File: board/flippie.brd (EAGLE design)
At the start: 98.3 x 55.7 mm, 28 parts, among them J1 INT_3V3, U1 FPF2702MX, U10 ULN2803ADW, U11 TD62783AP, U12 TD62783AP, U13 TD62783AP, U14 ULN2803ADW, U2 SN74AHC595D, U3 SN74AHC595D, U4 SN74AHC595D, U5 SN74AHC595D, U6 SN74AHC595D, U7 SN74AHC595D, U8 SN74AHC595D, U9 ULN2803ADW, X1 PWR, X2 BROSE-60-POL

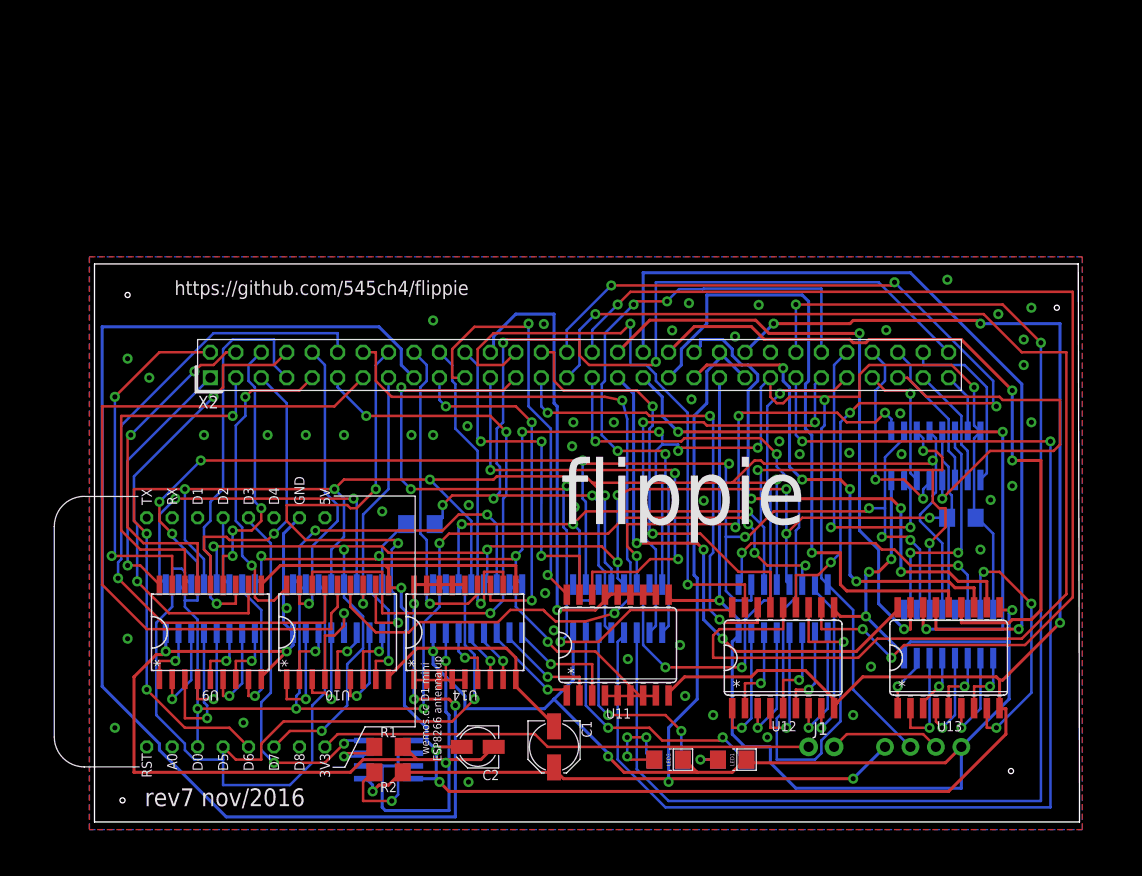
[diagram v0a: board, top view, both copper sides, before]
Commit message: Some clean-ups
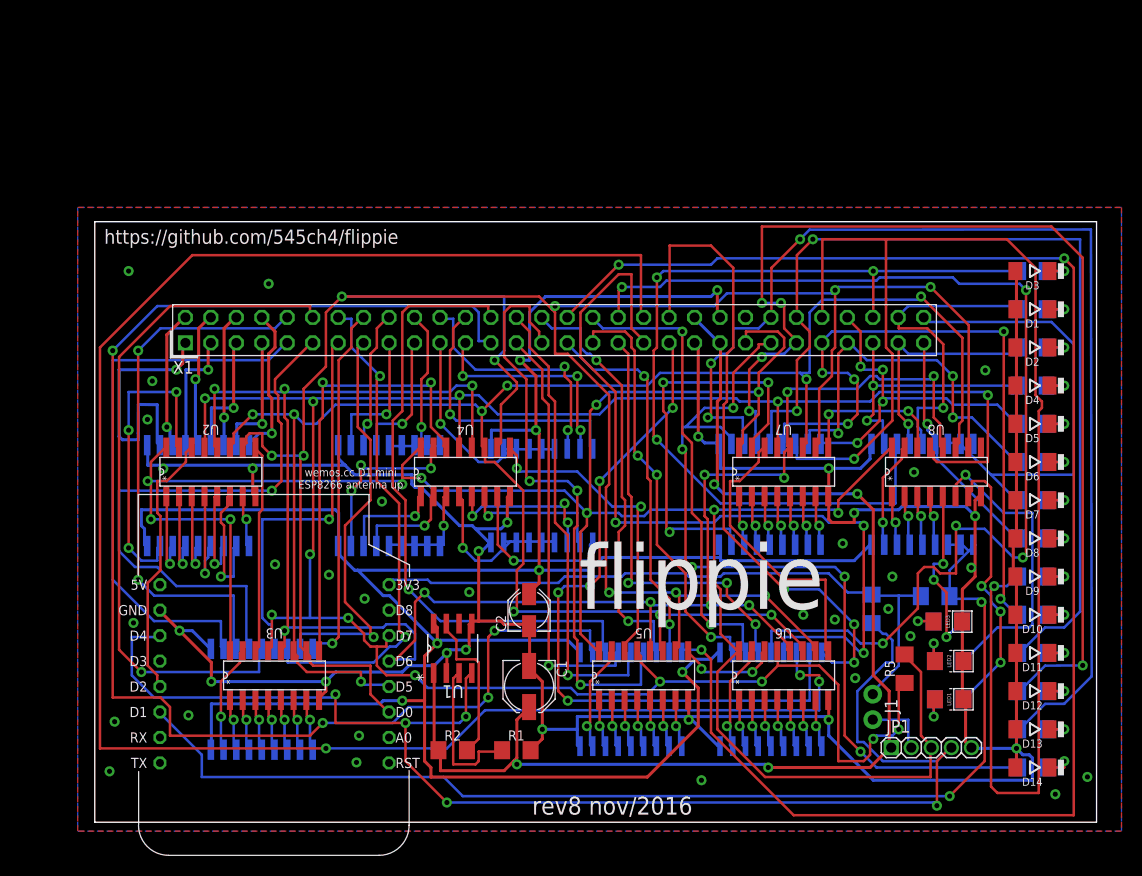
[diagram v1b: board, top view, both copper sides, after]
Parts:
- removed X2: BROSE-60-POL, con-panduit:057-060-1
- added D1, D10, D11, D12, D13, D14, D2, D3, D4, D5, D6, D7, D8, D9: BZV55, diode:SOD80C
- added JP1: (no value), pinhead:1_05X2MM
- added LED3: A, adafruit:1206
- added R10, R11, R12, R13, R14, R15, R16, R17, R18, R19, R20, R21, R22, R9: 100K, rcl:R1206
- added R7, R8: 150, rcl:R1206
- added U15, U16: TD62783AP, uln-udn:SO18W
- LED1: value A -> C
- R4: value 150 -> 10K
- X1: value PWR -> BROSE-60-POL; device adafruit:1X04-CLEANBIG -> con-panduit:057-060-1
- moved U13 76.6 mm to (10.3, 32.6), flipped to the bottom
- moved U9 56.3 mm to (67.5, 12.2), flipped to the bottom
- moved X1 55.5 mm to (45.9, 49.1)
- moved U12 52.2 mm to (16.7, 12.2), flipped to the bottom
- moved R5 50.4 mm to (80.8, 15.3), flipped to the top, turned to 270 degrees
- moved U8 34.6 mm to (84.0, 35.1), flipped to the top
- moved U10 30.0 mm to (53.5, 12.2), flipped to the bottom
- moved LED2 29.7 mm to (85.3, 16.1)
- moved R6 28.6 mm to (85.3, 12.2)
- moved U11 27.2 mm to (29.4, 32.6), flipped to the bottom
- moved LED1 22.5 mm to (85.3, 12.2)
- moved R4 20.5 mm to (77.5, 21.3), turned to 270 degrees
- moved MCU1 17.4 mm to (29.4, 23.7), turned to 180 degrees
- moved U6 17.0 mm to (68.8, 14.8), flipped to the top
- moved U14 15.6 mm to (44.6, 32.6), flipped to the bottom
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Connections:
- removed net SR10_ROW15_24V: U10.12, X2.15
- removed net SR11_ROW14_24V: U10.13, X2.14
- removed net SR12_ROW13_24V: U10.14, X2.13
- removed net SR13_ROW12_24V: U10.15, X2.12
- removed net SR14_ROW11_24V: U10.16, X2.11
- removed net SR15_ROW10_24V: U10.17, X2.10
- removed net SR16_ROW9_24V: U10.18, X2.9
- removed net SR17_ROW4_GND: U11.11, U11.12, U11.13, U11.14, U11.15, X2.24
- removed net SR18_ROW3_GND: U11.16, X2.23
- removed net SR19_ROW2_GND: U11.17, X2.22
- removed net SR1_ROW8_24V: U9.11, X2.8
- removed net SR20_ROW1_GND: U11.18, X2.21
- removed net SR21_ROW20_24V: U14.11, X2.20
- removed net SR22_ROW19_24V: U14.12, X2.19
- removed net SR23_ROW18_24V: U14.13, X2.18
- removed net SR24_ROW17_24V: U14.14, U14.15, U14.16, U14.17, U14.18, X2.17
- removed net SR25_ROW12_GND: U12.11, X2.32
- removed net SR26_ROW11_GND: U12.12, X2.31
- removed net SR27_ROW10_GND: U12.13, X2.30
- removed net SR28_ROW9_GND: U12.14, X2.29
- removed net SR29_ROW8_GND: U12.15, X2.28
- removed net SR2_ROW7_24V: U9.12, X2.7
- removed net SR30_ROW7_GND: U12.16, X2.27
- removed net SR31_ROW6_GND: U12.17, X2.26
- removed net SR32_ROW5_GND: U12.18, X2.25
- removed net SR33_ROW20_GND: U13.11, X2.40
- removed net SR34_ROW19_GND: U13.12, X2.39
- removed net SR35_ROW18_GND: U13.13, X2.38
- removed net SR36_ROW17_GND: U13.14, X2.37
- removed net SR37_ROW16_GND: U13.15, X2.36
- removed net SR38_ROW15_GND: U13.16, X2.35
- removed net SR39_ROW14_GND: U13.17, X2.34
- removed net SR3_ROW6_24V: U9.13, X2.6
- removed net SR40_ROW13_GND: U13.18, X2.33
- removed net SR41_ADDR7: U7.15, X2.59
- removed net SR42_ADDR6: U7.1, X2.58
- removed net SR43_ADDR5: U7.2, X2.57
- removed net SR44_ADDR4: U7.3, X2.56
- removed net SR45_ADDR3: U7.4, X2.55
- removed net SR46_ADDR2: U7.5, X2.54
- removed net SR47_ADDR1: U7.6, X2.53
- removed net SR48_B1@FP2800A: U7.7, X2.52
- removed net SR49_B0@FP2800A: U8.15, X2.51
- removed net SR4_ROW5_24V: U9.14, X2.5
- removed net SR50_A2@FP2800A: U8.1, X2.50
- removed net SR51_A1@FP2800A: U8.2, X2.49
- removed net SR52_A0@FP2800A: U8.3, X2.48
- removed net SR53_D@FP2800A: U8.4, X2.47
- removed net SR54_ADDR8_NOT_EN: R5.1, U8.5, X2.60
- removed net SR56_LED_A: R4.1, U8.7
- removed net SR5_ROW4_24V: U9.15, X2.4
- removed net SR6_ROW3_24V: U9.16, X2.3
- removed net SR7_ROW2_24V: U9.17, X2.2
- removed net SR8_ROW1_24V: U9.18, X2.1
- removed net SR9_ROW16_24V: U10.11, X2.16
- new net N$10: D6.C, R14.2
- new net N$12: D7.C, R15.2
- new net N$13: D8.C, R16.2
- new net N$14: D9.C, R17.2
- new net N$15: D10.C, R18.2
- new net N$16: D11.C, R19.2
- new net N$17: D12.C, R20.2
- new net N$18: D13.C, R21.2
- new net N$19: D14.C, R22.2
- new net N$2: D1.C, R9.2
- new net N$5: LED3.A, R8.2
- new net N$6: D2.C, R10.2
- new net N$7: D3.C, R11.2
- new net N$8: D4.C, R12.2
- new net N$9: D5.C, R13.2
- new net NOT_EN_ADDR8@FP2800A: MCU1.D1, R3.2, U15.1, U15.2, U15.3
- new net NOT_EN_ADDR8@FP2800A_VS: R15.1, U15.16, U15.17, U15.18, X1.60
- new net SR10_ROW10_SET: U12.12, X1.10
- new net SR11_ROW11_SET: U12.13, X1.11
- new net SR12_ROW12_SET: U12.14, X1.12
- new net SR13_ROW13_SET: U12.15, X1.13
- new net SR14_ROW14_SET: U12.16, X1.14
- new net SR15_ROW15_SET: U12.17, X1.15
- new net SR16_ROW16_SET: U12.18, X1.16
- new net SR17_ROW17_SET: U11.11, X1.17
- new net SR18_ROW18_SET: U11.12, X1.18
- new net SR19_ROW19_SET: U11.13, X1.19
- new net SR1_ROW1_SET: U13.11, X1.1
- new net SR20_ROW20_SET: U11.14, U11.15, U11.16, U11.17, U11.18, X1.20
- new net SR21_ROW1_RST: U14.11, U14.12, U14.13, U14.14, U14.15, X1.21
- new net SR22_ROW2_RST: U14.16, X1.22
- new net SR23_ROW3_RST: U14.17, X1.23
- new net SR24_ROW4_RST: U14.18, X1.24
- new net SR25_ROW5_RST: U10.11, X1.25
- new net SR26_ROW6_RST: U10.12, X1.26
- new net SR27_ROW7_RST: U10.13, X1.27
- new net SR28_ROW8_RST: U10.14, X1.28
- new net SR29_ROW9_RST: U10.15, X1.29
- new net SR2_ROW2_SET: U13.12, X1.2
- new net SR30_ROW10_RST: U10.16, X1.30
- new net SR31_ROW11_RST: U10.17, X1.31
- new net SR32_ROW12_RST: U10.18, X1.32
- new net SR33_ROW13_RST: U9.11, X1.33
- new net SR34_ROW14_RST: U9.12, X1.34
- new net SR35_ROW15_RST: U9.13, X1.35
- new net SR36_ROW16_RST: U9.14, X1.36
- new net SR37_ROW17_RST: U9.15, X1.37
- new net SR38_ROW18_RST: U9.16, X1.38
- new net SR39_ROW19_RST: U9.17, X1.39
- new net SR3_ROW3_SET: U13.13, X1.3
- new net SR40_ROW20_RST: U9.18, X1.40
- new net SR41_D@FP2800A: U16.8, U7.15
- new net SR41_D@FP2800A_VS: R22.1, U16.11, X1.47
- new net SR42_A0@FP2800A: U16.7, U7.1
- new net SR42_A0@FP2800A_VS: R21.1, U16.12, X1.48
- new net SR43_A1@FP2800A: U16.6, U7.2
- new net SR43_A1@FP2800A_VS: R20.1, U16.13, X1.49
- new net SR44_A2@FP2800A: U16.5, U7.3
- new net SR44_A2@FP2800A_VS: R19.1, U16.14, X1.50
- new net SR45_B0@FP2800A: U16.4, U7.4
- new net SR45_B0@FP2800A_VS: R18.1, U16.15, X1.51
- new net SR46_B1@FP2800A: U16.3, U7.5
- new net SR46_B1@FP2800A_VS: R17.1, U16.16, X1.52
- new net SR47_ADDR1@FP2800A: U16.2, U7.6
- new net SR47_ADDR1@FP2800A_VS: R14.1, U16.17, X1.53
- new net SR48_ADDR2@FP2800A: U16.1, U7.7
- new net SR48_ADDR2@FP2800A_VS: R13.1, U16.18, X1.54
- new net SR49_ADDR3@FP2800A: U15.8, U8.15
- new net SR49_ADDR3@FP2800A_VS: R12.1, U15.11, X1.55
- new net SR4_ROW4_SET: U13.14, X1.4
- new net SR50_ADDR4@FP2800A: U15.7, U8.1
- new net SR50_ADDR4@FP2800A_VS: R11.1, U15.12, X1.56
- new net SR51_ADDR5@FP2800A: U15.6, U8.2
- new net SR51_ADDR5@FP2800A_VS: R10.1, U15.13, X1.57
- new net SR52_ADDR6@FP2800A: U15.5, U8.3
- new net SR52_ADDR6@FP2800A_VS: R9.1, U15.14, X1.58
- new net SR53_ADDR7@FP2800A: U15.4, U8.4
- new net SR53_ADDR7@FP2800A_VS: R16.1, U15.15, X1.59
- new net SR54_LED_A: R8.1, U8.5
- new net SR56_LED_C: R6.1, U8.7
- new net SR5_ROW5_SET: U13.15, X1.5
- new net SR6_ROW6_SET: U13.16, X1.6
- new net SR7_ROW7_SET: U13.17, X1.7
- new net SR8_ROW8_SET: U13.18, X1.8
- new net SR9_ROW9_SET: U12.11, X1.9
- net +24V: now also JP1.1, X1.42, X1.43; no longer X1.1, X2.42, X2.43
- net +3V3: now also JP1.3; no longer X1.3
- net +3V3_SW: now also R3.1, R4.1
- net +5V: now also JP1.2, R5.1, X1.45; no longer R3.1, R5.2, X1.2, X2.45
- net +VS: now also U15.9, U16.9, X1.44; no longer X2.44
- net EN_VS: now also JP1.4, MCU1.D4, R4.2; no longer MCU1.D3
- net GND: now also D1.A, D10.A, D11.A, D12.A, D13.A, D14.A, D2.A, D3.A, D4.A, D5.A, D6.A, D7.A, D8.A, D9.A, JP1.5, LED3.C, U15.10, U16.10, X1.41; no longer X1.4, X2.41
- net N$142: now also R7.2; no longer R6.2
- net N$148: now also R6.2; no longer R4.2
- net SR1: now also U13.8; no longer U9.8
- net SR10: now also U12.7; no longer U10.7
- net SR11: now also U12.6; no longer U10.6
- net SR12: now also U12.5; no longer U10.5
- net SR13: now also U12.4; no longer U10.4
- net SR14: now also U12.3; no longer U10.3
- net SR15: now also U12.2; no longer U10.2
- net SR16: now also U12.1; no longer U10.1
- net SR17: no longer U11.4, U11.5, U11.6, U11.7
- net SR18: now also U11.7; no longer U11.3
- net SR19: now also U11.6; no longer U11.2
- net SR2: now also U13.7; no longer U9.7
- net SR20: now also U11.2, U11.3, U11.4, U11.5
- net SR21: now also U14.4, U14.5, U14.6, U14.7
- net SR22: now also U14.3; no longer U14.7
- net SR23: now also U14.2; no longer U14.6
- net SR24: no longer U14.2, U14.3, U14.4, U14.5
- net SR25: now also U10.8; no longer U12.8
- net SR26: now also U10.7; no longer U12.7
- net SR27: now also U10.6; no longer U12.6
- net SR28: now also U10.5; no longer U12.5
- net SR29: now also U10.4; no longer U12.4
- net SR3: now also U13.6; no longer U9.6
- net SR30: now also U10.3; no longer U12.3
- net SR31: now also U10.2; no longer U12.2
- net SR32: now also U10.1; no longer U12.1
- net SR33: now also U9.8; no longer U13.8
- net SR34: now also U9.7; no longer U13.7
- net SR35: now also U9.6; no longer U13.6
- net SR36: now also U9.5; no longer U13.5
- net SR37: now also U9.4; no longer U13.4
- net SR38: now also U9.3; no longer U13.3
- net SR39: now also U9.2; no longer U13.2
- net SR4: now also U13.5; no longer U9.5
- net SR40: now also U9.1; no longer U13.1
- net SR5: now also U13.4; no longer U9.4
- net SR55_LED_B: now also R7.1; no longer R6.1
- net SR6: now also U13.3; no longer U9.3
- net SR7: now also U13.2; no longer U9.2
- net SR8: now also U13.1; no longer U9.1
- net SR9: now also U12.8; no longer U10.8
- net ~OE: now also R5.2; no longer R3.2
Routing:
- net SR38_ROW18_RST: track 0.00 -> 185.5 mm, vias 0 -> 3
- net SR32_ROW12_RST: track 0.00 -> 158.5 mm, vias 0 -> 3
- net SR24_ROW17_24V: track 143.4 -> 0.00 mm, vias 3 -> 0
- net SR46_B1@FP2800A_VS: track 0.00 -> 142.0 mm, vias 0 -> 2
- net SR25_ROW5_RST: track 0.00 -> 138.4 mm, vias 0 -> 4
- net SR52_A0@FP2800A: track 131.8 -> 0.00 mm, vias 2 -> 0
- net SR28_ROW9_GND: track 129.7 -> 0.00 mm, vias 1 -> 0
- net SR53_D@FP2800A: track 126.0 -> 0.00 mm, vias 2 -> 0
- net NOT_EN_ADDR8@FP2800A: track 0.00 -> 116.8 mm, vias 0 -> 2
- net SR42_A0@FP2800A_VS: track 0.00 -> 113.2 mm, vias 0 -> 3
- net SR25_ROW12_GND: track 113.2 -> 0.00 mm, vias 3 -> 0
- net SR36_ROW16_RST: track 0.00 -> 110.5 mm, vias 0 -> 5
- net SR43_A1@FP2800A_VS: track 0.00 -> 109.6 mm, vias 0 -> 5
- net SR54_ADDR8_NOT_EN: track 106.2 -> 0.00 mm, vias 5 -> 0
- net EN_VS: track 36.4 -> 139.3 mm, vias 2 -> 5
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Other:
- board size 98.3 x 55.7 mm -> 99.9 x 59.9 mm
- board text added: "EN+"
- board text added: "rev8 nov/2016"
- board text removed: "rev7 nov/2016"

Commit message: Update board to rev10
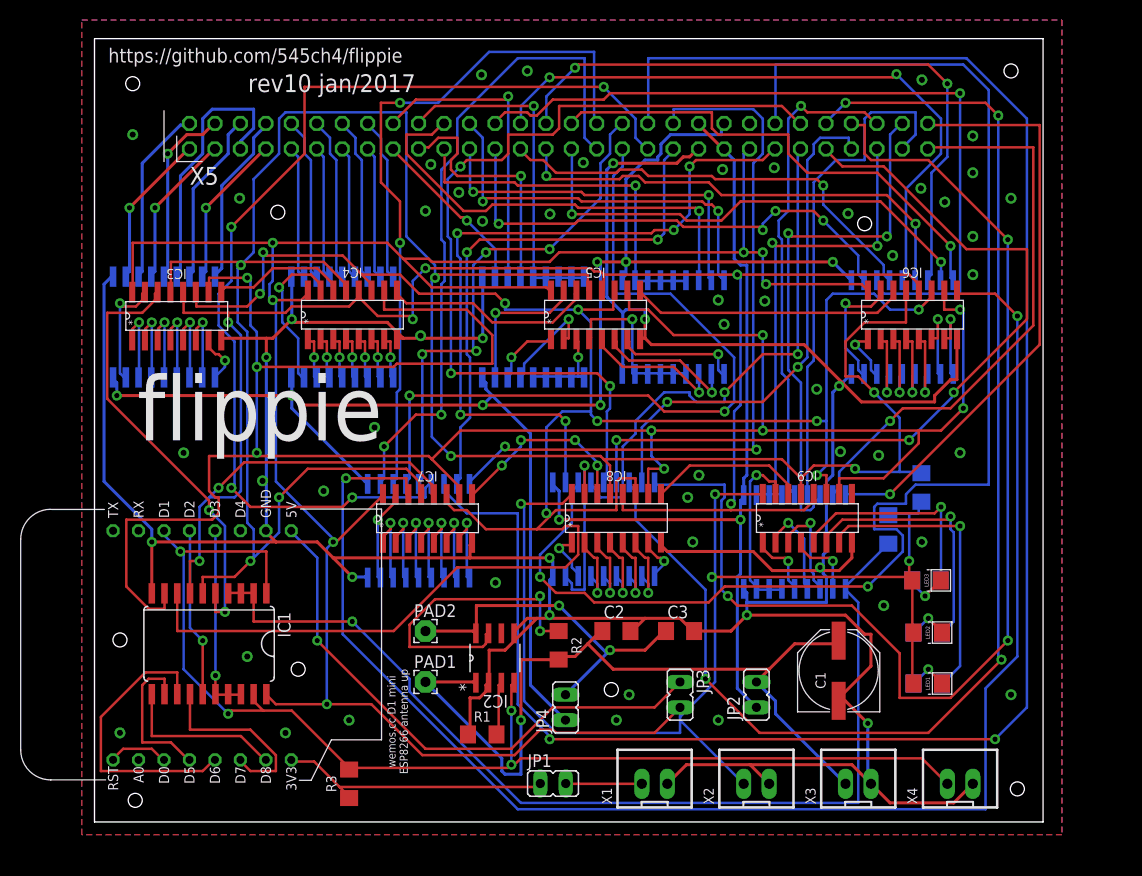
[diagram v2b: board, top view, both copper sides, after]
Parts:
- removed D1, D10, D11, D12, D13, D14, D2, D3, D4, D5, D6, D7, D8, D9: BZV55, diode:SOD80C
- removed J1: INT_3V3, SparkFun-Connectors:1X02_NO_SILK
- removed R10, R11, R12, R13, R14, R15, R16, R17, R18, R19, R20, R21, R22, R9: 100K, rcl:R1206
- removed U1: FPF2702MX, ON Semiconductor_By_element14_Batch_1:SOIC127P600X175-8N
- removed U10, U14, U9: ULN2803ADW, Texas Instruments_By_element14_Batch_1:SOIC127P1030X265-18N
- removed U11, U12, U13, U15, U16: TD62783AP, uln-udn:SO18W
- removed U2, U3, U4, U5, U6, U7, U8: SN74AHC595D, Texas Instruments_By_element14_Batch_1:SOIC127P600X175-16N
- added C3: 22u, rcl:C1206
- added IC1: 74HCT245DW, 74xx-eu:SO20W
- added IC10, IC11, IC12: TD62783AFG, uln-udn:SO18W
- added IC13, IC14, IC15, IC16, IC17: ULN2803A, Texas Instruments_By_element14_Batch_1:SOIC127P1030X265-18N
- added IC2: FPF2702MX, ON Semiconductor_By_element14_Batch_1:SOIC127P600X175-8N
- added IC3, IC4, IC5, IC6, IC7, IC8, IC9: SN74AHC595D, Texas Instruments_By_element14_Batch_1:SOIC127P600X175-16N
- added JP2: 24V, jumper:JP1
- added JP3: 5V, jumper:JP1
- added JP4: VS, jumper:JP1
- added PAD1: 24V, wirepad:2,15/1,0
- added PAD2: VS, wirepad:2,15/1,0
- added X2: 5V, Rembrandt Electronics - JST XH Connectors v1-0:JST-XH-02-PACKAGE-LONG-PAD
- added X3: 24V, Rembrandt Electronics - JST XH Connectors v1-0:JST-XH-02-PACKAGE-LONG-PAD
- added X4: ~EN_PWR, Rembrandt Electronics - JST XH Connectors v1-0:JST-XH-02-PACKAGE-LONG-PAD
- added X5: BROSE-60-POL, con-panduit:057-060-1
- C1: value 100u -> 100u/35V; device rcl:PANASONIC_C -> rcl:PANASONIC_E
- C2: value 22u -> 100u; device rcl:PANASONIC_B -> rcl:C1206
- JP1: value (none) -> 3V3; device pinhead:1_05X2MM -> jumper:JP1
- LED1: value C -> C (red)
- LED2: value B -> B (yellow)
- LED3: value A -> A (green)
- R1: value 680K -> 470K
- R6: value 150 -> 180
- R8: value 150 -> 120
- X1: value BROSE-60-POL -> 3V3; device con-panduit:057-060-1 -> Rembrandt Electronics - JST XH Connectors v1-0:JST-XH-02-PACKAGE-LONG-PAD
- moved R3 61.4 mm to (25.4, 3.81), flipped to the top, turned to 90 degrees
- moved X1 46.4 mm to (55.9, 3.81)
- moved JP1 37.9 mm to (45.7, 3.84), turned to 270 degrees
- moved C1 30.9 mm to (74.2, 15.1), turned to 90 degrees
- moved MCU1 20.0 mm to (19.6, 6.20), turned to 90 degrees
- moved R5 18.2 mm to (82.5, 33.4), flipped to the bottom, turned to 90 degrees
- moved R2 14.9 mm to (46.3, 17.6), turned to 270 degrees
- moved C2 8.96 mm to (52.1, 19.1), turned to 0 degrees
- moved R4 8.10 mm to (79.2, 29.2)
- moved LED3 4.64 mm to (83.0, 24.1)
- moved R8 4.64 mm to (83.0, 24.1)
- moved R1 3.75 mm to (38.7, 8.74), turned to 0 degrees
- moved LED2 3.56 mm to (83.1, 18.9)
- moved R7 3.56 mm to (83.1, 18.9)
- moved LED1 2.65 mm to (83.1, 13.8)
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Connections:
- removed net +24V: C1.+, JP1.1, R2.2, U1.1, X1.42, X1.43
- removed net +3V3: J1.2, JP1.3
- removed net +3V3_SW: J1.1, MCU1.3V3, R3.1, R4.1
- removed net +5V: JP1.2, R5.1, U2.16, U3.16, U4.16, U5.16, U6.16, U7.16, U8.16, X1.45
- removed net +VS: C2.+, U1.8, U10.10, U11.9, U12.9, U13.9, U14.10, U15.9, U16.9, U9.10, X1.44
- removed net EN_VS: JP1.4, MCU1.D4, R4.2, U1.4
- removed net N$10: D6.C, R14.2
- removed net N$12: D7.C, R15.2
- removed net N$13: D8.C, R16.2
- removed net N$14: D9.C, R17.2
- removed net N$142: LED2.A, R7.2
- removed net N$148: LED1.A, R6.2
- removed net N$15: D10.C, R18.2
- removed net N$16: D11.C, R19.2
- removed net N$17: D12.C, R20.2
- removed net N$18: D13.C, R21.2
- removed net N$19: D14.C, R22.2
- removed net N$2: D1.C, R9.2
- removed net N$41: U7.9, U8.14
- removed net N$6: D2.C, R10.2
- removed net N$9: D5.C, R13.2
- removed net NOT_EN_ADDR8@FP2800A: MCU1.D1, R3.2, U15.1, U15.2, U15.3
- removed net NOT_EN_ADDR8@FP2800A_VS: R15.1, U15.16, U15.17, U15.18, X1.60
- removed net SR41_D@FP2800A_VS: R22.1, U16.11, X1.47
- removed net SR42_A0@FP2800A_VS: R21.1, U16.12, X1.48
- removed net SR43_A1@FP2800A_VS: R20.1, U16.13, X1.49
- removed net SR44_A2@FP2800A_VS: R19.1, U16.14, X1.50
- removed net SR45_B0@FP2800A_VS: R18.1, U16.15, X1.51
- removed net SR46_B1@FP2800A_VS: R17.1, U16.16, X1.52
- removed net SR47_ADDR1@FP2800A_VS: R14.1, U16.17, X1.53
- removed net SR48_ADDR2@FP2800A_VS: R13.1, U16.18, X1.54
- removed net SR49_ADDR3@FP2800A_VS: R12.1, U15.11, X1.55
- removed net SR50_ADDR4@FP2800A_VS: R11.1, U15.12, X1.56
- removed net SR51_ADDR5@FP2800A_VS: R10.1, U15.13, X1.57
- removed net SR52_ADDR6@FP2800A_VS: R9.1, U15.14, X1.58
- removed net SR53_ADDR7@FP2800A_VS: R16.1, U15.15, X1.59
- new net 24V: IC16.10, IC17.10, JP2.1, X5.42, X5.43
- new net 24V_SW: C1.+, C2.1, IC2.1, JP2.2, PAD1.1, R2.2, X3.1
- new net 3V3: JP1.2, X1.1
- new net 3V3_SW: JP1.1, MCU1.3V3, R3.1
- new net N$21: LED2.C, R7.2
- new net N$23: LED3.C, R8.2
- new net RCLK_5V: IC1.7, IC3.12, IC4.12, IC5.12, IC6.12, IC7.12, IC8.12, IC9.12
- new net SER_5V: IC1.5, IC3.14
- new net SR41_D@FP2800A_24V: IC17.11, X5.47
- new net SR42_A0@FP2800A_24V: IC17.12, X5.48
- new net SR43_A1@FP2800A_24V: IC17.13, X5.49
- new net SR44_A2@FP2800A_24V: IC17.14, X5.50
- new net SR45_B0@FP2800A_24V: IC17.15, X5.51
- new net SR46_B1@FP2800A_24V: IC17.16, X5.52
- new net SR47_ADDR1@FP2800A_24V: IC17.17, X5.53
- new net SR48_ADDR2@FP2800A_24V: IC17.18, X5.54
- new net SR49_ADDR3@FP2800A_24V: IC16.11, IC16.12, IC16.13, X5.55
- new net SR50_ADDR4@FP2800A_24V: IC16.14, X5.56
- new net SR51_ADDR5@FP2800A_24V: IC16.15, X5.57
- new net SR52_ADDR6@FP2800A_24V: IC16.16, X5.58
- new net SR53_ADDR7@FP2800A_24V: IC16.17, X5.59
- new net SRCLK_5V: IC1.8, IC3.11, IC4.11, IC5.11, IC6.11, IC7.11, IC8.11, IC9.11
- new net VCC: IC1.20, IC3.16, IC4.16, IC5.16, IC6.16, IC7.16, IC8.16, IC9.16, JP3.2, LED1.A, LED2.A, LED3.A, R4.1, R5.1, X2.1, X5.45
- new net VCC_SW: JP3.1, MCU1.5V
- new net VS: IC10.9, IC11.9, IC12.9, IC13.10, IC14.10, IC15.10, JP4.1, X5.44
- new net VS_SW: C3.1, IC2.8, JP4.2, PAD2.1
- new net ~EN_ADDR8@FP2800A: IC1.16, IC1.17, IC1.18, MCU1.D3
- new net ~EN_ADDR8@FP2800A_24V: IC16.18, X5.60
- new net ~EN_ADDR8@FP2800A_5V: IC1.2, IC1.3, IC1.4, IC16.1, R4.2
- new net ~EN_POWER_RAILS: IC1.1, IC1.19, IC2.4, MCU1.D1, R3.2, X4.1
- new net ~OE_5V: IC1.6, IC3.13, IC4.13, IC5.13, IC6.13, IC7.13, IC8.13, IC9.13, R5.2
- new net ~SRCLR_5V: IC1.9, IC3.10, IC4.10, IC5.10, IC6.10, IC7.10, IC8.10, IC9.10
- net GND: now also C2.2, C3.2, IC1.10, IC10.10, IC11.10, IC12.10, IC13.9, IC14.9, IC15.9, IC16.9, IC17.9, IC2.2, IC2.5, IC3.8, IC4.8, IC5.8, IC6.8, IC7.8, IC8.8, IC9.8, X1.2, X2.2, X3.2, X4.2, X5.41; no longer C2.-, D1.A, D10.A, D11.A, D12.A, D13.A, D14.A, D2.A, D3.A, D4.A, D5.A, D6.A, D7.A, D8.A, D9.A, JP1.5, LED1.C, LED2.C, LED3.C, U1.2, U1.5, U10.9, U11.10, U12.10, U13.10, U14.9, U15.10, U16.10, U2.8, U3.8, U4.8, U5.8, U6.8, U7.8, U8.8, U9.9, X1.41
- net N$1: now also IC6.9, IC7.14; no longer U5.9, U6.14
- net N$11: now also IC4.9, IC5.14; no longer U3.9, U4.14
- net N$22: now also IC5.9, IC6.14; no longer U4.9, U5.14
- net N$3: now also IC2.7; no longer U1.7
- net N$31: now also IC3.9, IC4.14; no longer U2.9, U3.14
- net N$37: now also IC7.9, IC8.14; no longer U6.9, U7.14
- net N$4: now also IC2.3; no longer U1.3
- net N$5: now also LED1.C, R6.2; no longer LED3.A, R8.2
- net N$7: now also IC8.9, IC9.14; no longer D3.C, R11.2
- net N$8: now also MCU1.D0, MCU1.RST; no longer D4.C, R12.2
- net RCLK: now also IC1.13; no longer U2.12, U3.12, U4.12, U5.12, U6.12, U7.12, U8.12
- net SER: now also IC1.15; no longer U2.14
- net SR1: now also IC12.8, IC3.15; no longer U13.8, U2.15
- net SR10: now also IC11.7, IC4.1; no longer U12.7, U3.1
- net SR10_ROW10_SET: now also IC11.12, X5.10; no longer U12.12, X1.10
- net SR11: now also IC11.6, IC4.2; no longer U12.6, U3.2
- net SR11_ROW11_SET: now also IC11.13, X5.11; no longer U12.13, X1.11
- net SR12: now also IC11.5, IC4.3; no longer U12.5, U3.3
- net SR12_ROW12_SET: now also IC11.14, X5.12; no longer U12.14, X1.12
- net SR13: now also IC11.4, IC4.4; no longer U12.4, U3.4
- net SR13_ROW13_SET: now also IC11.15, X5.13; no longer U12.15, X1.13
- net SR14: now also IC11.3, IC4.5; no longer U12.3, U3.5
- net SR14_ROW14_SET: now also IC11.16, X5.14; no longer U12.16, X1.14
- net SR15: now also IC11.2, IC4.6; no longer U12.2, U3.6
- net SR15_ROW15_SET: now also IC11.17, X5.15; no longer U12.17, X1.15
- net SR16: now also IC11.1, IC4.7; no longer U12.1, U3.7
- net SR16_ROW16_SET: now also IC11.18, X5.16; no longer U12.18, X1.16
- net SR17: now also IC10.8, IC5.15; no longer U11.8, U4.15
- net SR17_ROW17_SET: now also IC10.11, X5.17; no longer U11.11, X1.17
- net SR18: now also IC10.7, IC5.1; no longer U11.7, U4.1
- net SR18_ROW18_SET: now also IC10.12, X5.18; no longer U11.12, X1.18
- net SR19: now also IC10.6, IC5.2; no longer U11.6, U4.2
- net SR19_ROW19_SET: now also IC10.13, X5.19; no longer U11.13, X1.19
- net SR1_ROW1_SET: now also IC12.11, X5.1; no longer U13.11, X1.1
- net SR2: now also IC12.7, IC3.1; no longer U13.7, U2.1
- net SR20: now also IC10.1, IC10.2, IC10.3, IC10.4, IC10.5, IC5.3; no longer U11.1, U11.2, U11.3, U11.4, U11.5, U4.3
- net SR20_ROW20_SET: now also IC10.14, IC10.15, IC10.16, IC10.17, IC10.18, X5.20; no longer U11.14, U11.15, U11.16, U11.17, U11.18, X1.20
- net SR21: now also IC15.4, IC15.5, IC15.6, IC15.7, IC15.8, IC5.4; no longer U14.4, U14.5, U14.6, U14.7, U14.8, U4.4
- net SR21_ROW1_RST: now also IC15.11, IC15.12, IC15.13, IC15.14, IC15.15, X5.21; no longer U14.11, U14.12, U14.13, U14.14, U14.15, X1.21
- net SR22: now also IC15.3, IC5.5; no longer U14.3, U4.5
- net SR22_ROW2_RST: now also IC15.16, X5.22; no longer U14.16, X1.22
- net SR23: now also IC15.2, IC5.6; no longer U14.2, U4.6
- net SR23_ROW3_RST: now also IC15.17, X5.23; no longer U14.17, X1.23
- net SR24: now also IC15.1, IC5.7; no longer U14.1, U4.7
- net SR24_ROW4_RST: now also IC15.18, X5.24; no longer U14.18, X1.24
- net SR25: now also IC14.8, IC6.15; no longer U10.8, U5.15
- net SR25_ROW5_RST: now also IC14.11, X5.25; no longer U10.11, X1.25
- net SR26: now also IC14.7, IC6.1; no longer U10.7, U5.1
- net SR26_ROW6_RST: now also IC14.12, X5.26; no longer U10.12, X1.26
- net SR27: now also IC14.6, IC6.2; no longer U10.6, U5.2
- net SR27_ROW7_RST: now also IC14.13, X5.27; no longer U10.13, X1.27
- net SR28: now also IC14.5, IC6.3; no longer U10.5, U5.3
- net SR28_ROW8_RST: now also IC14.14, X5.28; no longer U10.14, X1.28
- net SR29: now also IC14.4, IC6.4; no longer U10.4, U5.4
- net SR29_ROW9_RST: now also IC14.15, X5.29; no longer U10.15, X1.29
- net SR2_ROW2_SET: now also IC12.12, X5.2; no longer U13.12, X1.2
- net SR3: now also IC12.6, IC3.2; no longer U13.6, U2.2
- net SR30: now also IC14.3, IC6.5; no longer U10.3, U5.5
- net SR30_ROW10_RST: now also IC14.16, X5.30; no longer U10.16, X1.30
- net SR31: now also IC14.2, IC6.6; no longer U10.2, U5.6
- net SR31_ROW11_RST: now also IC14.17, X5.31; no longer U10.17, X1.31
- net SR32: now also IC14.1, IC6.7; no longer U10.1, U5.7
- net SR32_ROW12_RST: now also IC14.18, X5.32; no longer U10.18, X1.32
- net SR33: now also IC13.8, IC7.15; no longer U6.15, U9.8
- net SR33_ROW13_RST: now also IC13.11, X5.33; no longer U9.11, X1.33
- net SR34: now also IC13.7, IC7.1; no longer U6.1, U9.7
- net SR34_ROW14_RST: now also IC13.12, X5.34; no longer U9.12, X1.34
- net SR35: now also IC13.6, IC7.2; no longer U6.2, U9.6
- net SR35_ROW15_RST: now also IC13.13, X5.35; no longer U9.13, X1.35
- net SR36: now also IC13.5, IC7.3; no longer U6.3, U9.5
- net SR36_ROW16_RST: now also IC13.14, X5.36; no longer U9.14, X1.36
- net SR37: now also IC13.4, IC7.4; no longer U6.4, U9.4
- net SR37_ROW17_RST: now also IC13.15, X5.37; no longer U9.15, X1.37
- net SR38: now also IC13.3, IC7.5; no longer U6.5, U9.3
- net SR38_ROW18_RST: now also IC13.16, X5.38; no longer U9.16, X1.38
- net SR39: now also IC13.2, IC7.6; no longer U6.6, U9.2
- net SR39_ROW19_RST: now also IC13.17, X5.39; no longer U9.17, X1.39
- net SR3_ROW3_SET: now also IC12.13, X5.3; no longer U13.13, X1.3
- net SR4: now also IC12.5, IC3.3; no longer U13.5, U2.3
- net SR40: now also IC13.1, IC7.7; no longer U6.7, U9.1
- net SR40_ROW20_RST: now also IC13.18, X5.40; no longer U9.18, X1.40
- net SR41_D@FP2800A: now also IC17.8, IC8.15; no longer U16.8, U7.15
- net SR42_A0@FP2800A: now also IC17.7, IC8.1; no longer U16.7, U7.1
- net SR43_A1@FP2800A: now also IC17.6, IC8.2; no longer U16.6, U7.2
- net SR44_A2@FP2800A: now also IC17.5, IC8.3; no longer U16.5, U7.3
- net SR45_B0@FP2800A: now also IC17.4, IC8.4; no longer U16.4, U7.4
- net SR46_B1@FP2800A: now also IC17.3, IC8.5; no longer U16.3, U7.5
- net SR47_ADDR1@FP2800A: now also IC17.2, IC8.6; no longer U16.2, U7.6
- net SR48_ADDR2@FP2800A: now also IC17.1, IC8.7; no longer U16.1, U7.7
- net SR49_ADDR3@FP2800A: now also IC16.6, IC16.7, IC16.8, IC9.15; no longer U15.8, U8.15
- net SR4_ROW4_SET: now also IC12.14, X5.4; no longer U13.14, X1.4
- net SR5: now also IC12.4, IC3.4; no longer U13.4, U2.4
- net SR50_ADDR4@FP2800A: now also IC16.5, IC9.1; no longer U15.7, U8.1
- net SR51_ADDR5@FP2800A: now also IC16.4, IC9.2; no longer U15.6, U8.2
- net SR52_ADDR6@FP2800A: now also IC16.3, IC9.3; no longer U15.5, U8.3
- net SR53_ADDR7@FP2800A: now also IC16.2, IC9.4; no longer U15.4, U8.4
- net SR54_LED_A: now also IC9.5; no longer U8.5
- net SR55_LED_B: now also IC9.6; no longer U8.6
- net SR56_LED_C: now also IC9.7; no longer U8.7
- net SR5_ROW5_SET: now also IC12.15, X5.5; no longer U13.15, X1.5
- net SR6: now also IC12.3, IC3.5; no longer U13.3, U2.5
- net SR6_ROW6_SET: now also IC12.16, X5.6; no longer U13.16, X1.6
- net SR7: now also IC12.2, IC3.6; no longer U13.2, U2.6
- net SR7_ROW7_SET: now also IC12.17, X5.7; no longer U13.17, X1.7
- net SR8: now also IC12.1, IC3.7; no longer U13.1, U2.7
- net SR8_ROW8_SET: now also IC12.18, X5.8; no longer U13.18, X1.8
- net SR9: now also IC11.8, IC4.15; no longer U12.8, U3.15
- net SR9_ROW9_SET: now also IC11.11, X5.9; no longer U12.11, X1.9
- net SRCLK: now also IC1.12; no longer U2.11, U3.11, U4.11, U5.11, U6.11, U7.11, U8.11
- net ~OE: now also IC1.14; no longer R5.2, U2.13, U3.13, U4.13, U5.13, U6.13, U7.13, U8.13
- net ~SRCLR: now also IC1.11, MCU1.D8; no longer MCU1.D0, U2.10, U3.10, U4.10, U5.10, U6.10, U7.10, U8.10
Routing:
- net VCC: track 0.00 -> 339.9 mm, vias 0 -> 11
- net +VS: track 251.2 -> 0.00 mm, vias 7 -> 0
- net ~OE_5V: track 0.00 -> 246.9 mm, vias 0 -> 7
- net +5V: track 234.8 -> 0.00 mm, vias 10 -> 0
- net ~SRCLR_5V: track 0.00 -> 234.5 mm, vias 0 -> 9
- net ~SRCLR: track 247.9 -> 16.5 mm, vias 10 -> 0
- net SRCLK_5V: track 0.00 -> 216.4 mm, vias 0 -> 9
- net ~OE: track 225.9 -> 18.8 mm, vias 13 -> 0
- net RCLK_5V: track 0.00 -> 189.7 mm, vias 0 -> 7
- net SRCLK: track 198.6 -> 15.1 mm, vias 10 -> 0
- net VS: track 0.00 -> 167.4 mm, vias 0 -> 7
- net RCLK: track 190.6 -> 28.9 mm, vias 12 -> 0
- net N$1: track 10.1 -> 152.7 mm
- net SR46_B1@FP2800A_VS: track 142.0 -> 0.00 mm, vias 2 -> 0
- net EN_VS: track 139.3 -> 0.00 mm, vias 5 -> 0
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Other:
- board size 99.9 x 59.9 mm -> 94.6 x 78.2 mm
- board text added: "rev10 jan/2017"
- board text removed: "24V"
- board text removed: "3V3"
- board text removed: "5V0"
- board text removed: "EN+"
- board text removed: "GND"
- board text removed: "rev8 nov/2016"
